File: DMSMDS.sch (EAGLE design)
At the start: 11 parts, among them IC1 LM1117MPX-5.0

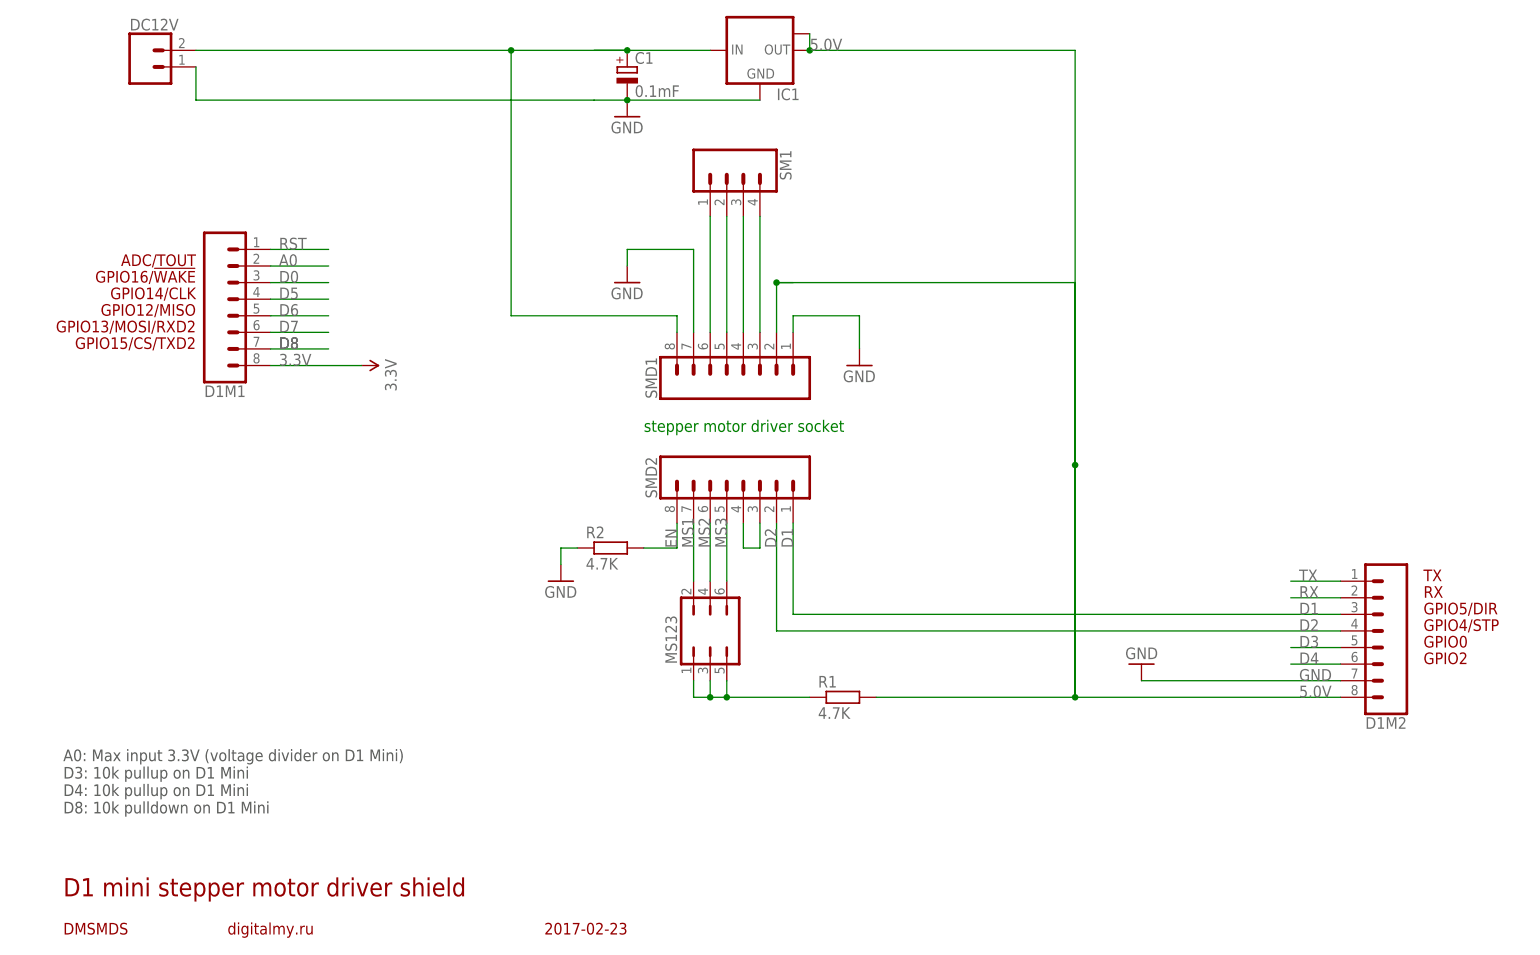
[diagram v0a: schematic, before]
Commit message: v1
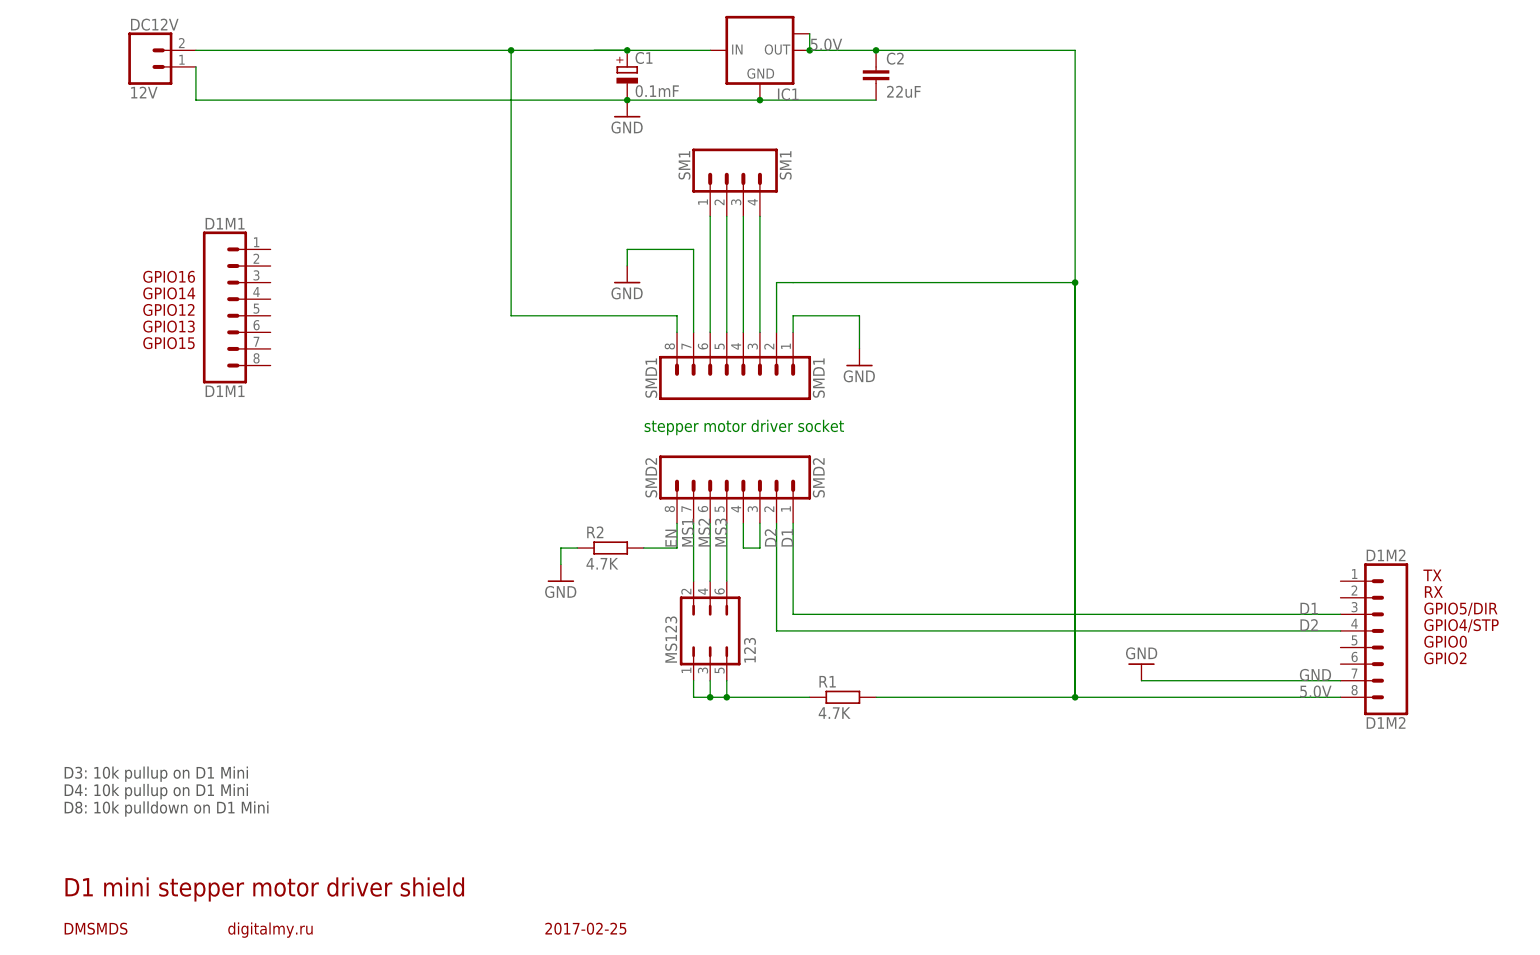
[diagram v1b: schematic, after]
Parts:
- added C2: 22uF, resistor:C-EUC1206
- D1M1: value (none) -> D1M1
- D1M2: value (none) -> D1M2
- DC12V: value (none) -> 12V
- MS123: value (none) -> 123
- SM1: value (none) -> SM1
- SMD1: value (none) -> SMD1
- SMD2: value (none) -> SMD2
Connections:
- net N$8 renamed MSP
- removed net 3.3V: D1M1.8
- removed net A0: D1M1.2
- removed net D0: D1M1.3
- removed net D3: D1M2.5
- removed net D4: D1M2.6
- removed net D5: D1M1.4
- removed net D6: D1M1.5
- removed net D7: D1M1.6
- removed net D8: D1M1.7
- removed net RST: D1M1.1
- removed net RX: D1M2.2
- removed net TX: D1M2.1
- net 5.0V: now also C2.1
- net GND: now also C2.2
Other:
- note added: "2017-02-25"
- note added: "D3: 10k pullup on D1 Mini D4: 10k pullup on D1 Mini D8: 10k pulldown on D1 Mini"
- note added: "GPIO12"
- note added: "GPIO13"
- note added: "GPIO14"
- note added: "GPIO15"
- note added: "GPIO16"
- note removed: "2017-02-23"
- note removed: "A0: Max input 3.3V (voltage divider on D1 Mini) D3: 10k pullup on D1 Mini D4: 10k pullup on D1 Mini D8: 10k pulldown on D1 Mini"
- note removed: "ADC/TOUT"
- note removed: "GPIO12/MISO"
- note removed: "GPIO13/MOSI/RXD2"
- note removed: "GPIO14/CLK"
- note removed: "GPIO15/CS/TXD2"
- note removed: "GPIO16/!WAKE"
